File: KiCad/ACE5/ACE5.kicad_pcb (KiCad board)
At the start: 2 copper layers, 160 x 100 mm, 99 parts, among them Q1 2N3904, Q3 BC237, U1 LM7805_TO220, X1 CRYSTALHC49U-V 6.556MHz, X2 5MHz

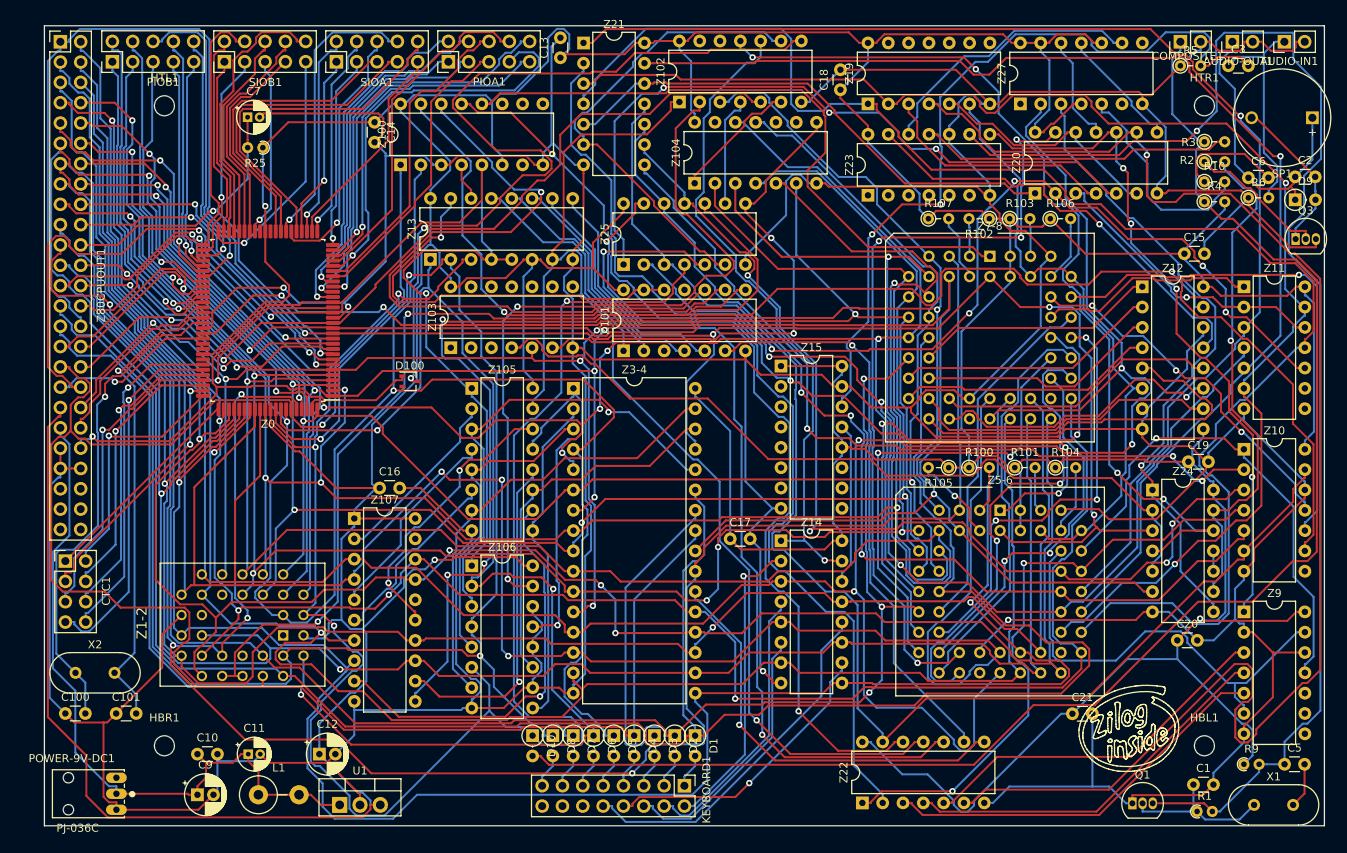
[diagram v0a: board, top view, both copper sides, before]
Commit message: Improve consitancy.
Signed-off-by: John Bradley <flypie@rocketmail.com>
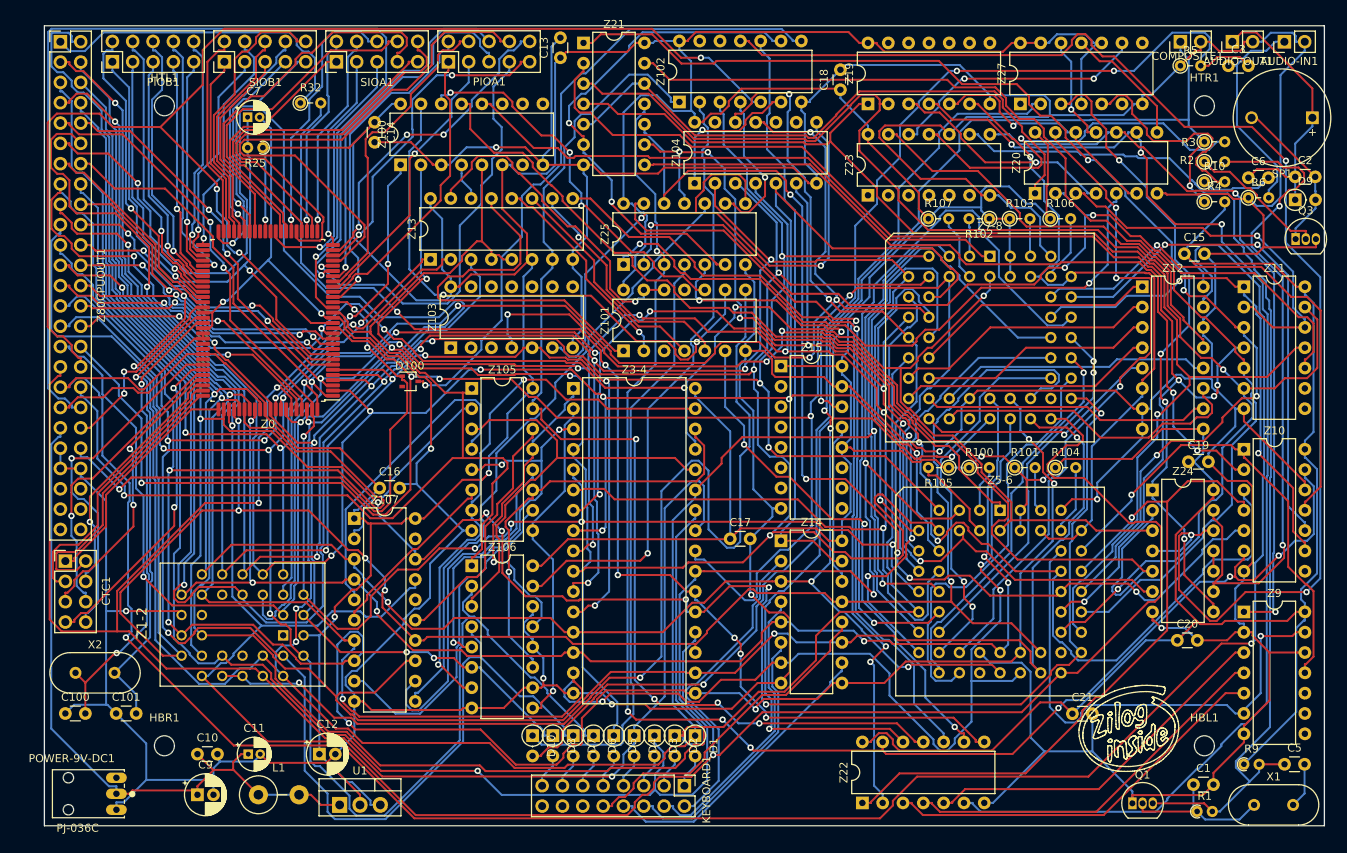
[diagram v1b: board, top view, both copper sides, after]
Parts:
- added R32: 1K0, Resistor_THT:R_Axial_DIN0204_L3.6mm_D1.6mm_P2.54mm_Vertical, F.Cu at (32.0, 9.65)
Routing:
- net #CPUCLK: track 161.4 -> 285.1 mm, vias 4 -> 2
- net Net-(R32-Pad2): track 52.8 -> 150.7 mm, vias 1 -> 6
- net //HALT: track 45.2 -> 131.5 mm, vias 2 -> 1
- net /A6: track 223.0 -> 302.3 mm, vias 3 -> 8
- net //WR: track 267.2 -> 194.9 mm, vias 4 -> 6
- net //IOREQ: track 106.9 -> 170.1 mm, vias 2 -> 3
- net /DA6: track 253.4 -> 313.1 mm, vias 4 -> 3
- net //RD: track 219.5 -> 276.4 mm, vias 3 -> 6
- net Net-(Z102-Pad11): track 115.8 -> 170.3 mm, vias 4 -> 3
- net /DA0: track 348.2 -> 294.4 mm, vias 4 -> 7
- net /A1: track 243.6 -> 294.1 mm, vias 6 -> 8
- net +5V: track 896.3 -> 847.2 mm, vias 3 -> 5
- net /A15: track 184.3 -> 135.6 mm, vias 4 -> 5
- net Net-(Z5-6-Pad17): track 44.5 -> 90.5 mm, vias 0 -> 1
- net /DA5: track 230.9 -> 274.4 mm, vias 2 -> 5
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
